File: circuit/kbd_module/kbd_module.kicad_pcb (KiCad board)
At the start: 2 copper layers, 50 x 50 mm, 25 parts, among them SW1 SW_SIMPLE, SW10 SW_SIMPLE, SW11 SW_SIMPLE, SW12 SW_SIMPLE, SW2 SW_SIMPLE, SW3 SW_SIMPLE, SW4 SW_SIMPLE, SW5 SW_SIMPLE, SW6 SW_SIMPLE, SW7 SW_SIMPLE, SW8 SW_SIMPLE, SW9 SW_SIMPLE, U1 NRF24LE1_PROG

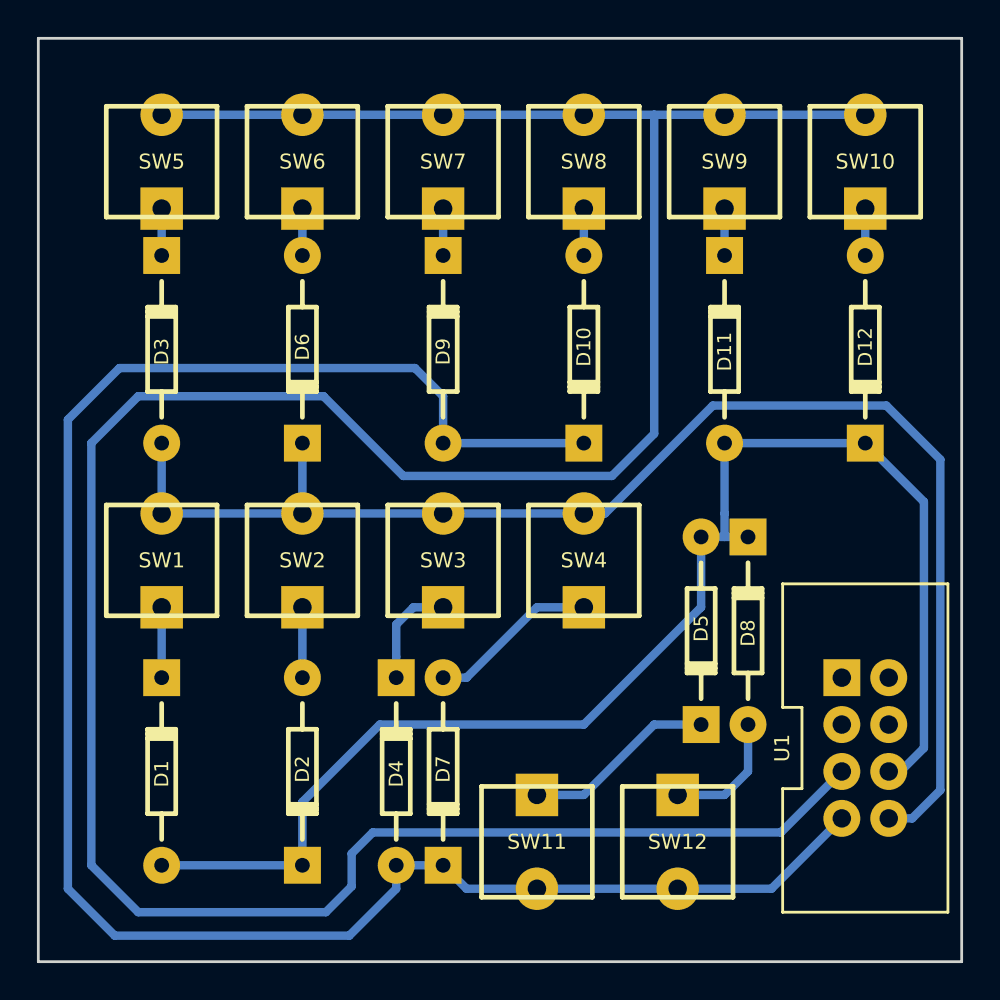
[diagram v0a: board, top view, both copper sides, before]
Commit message: dual diodes
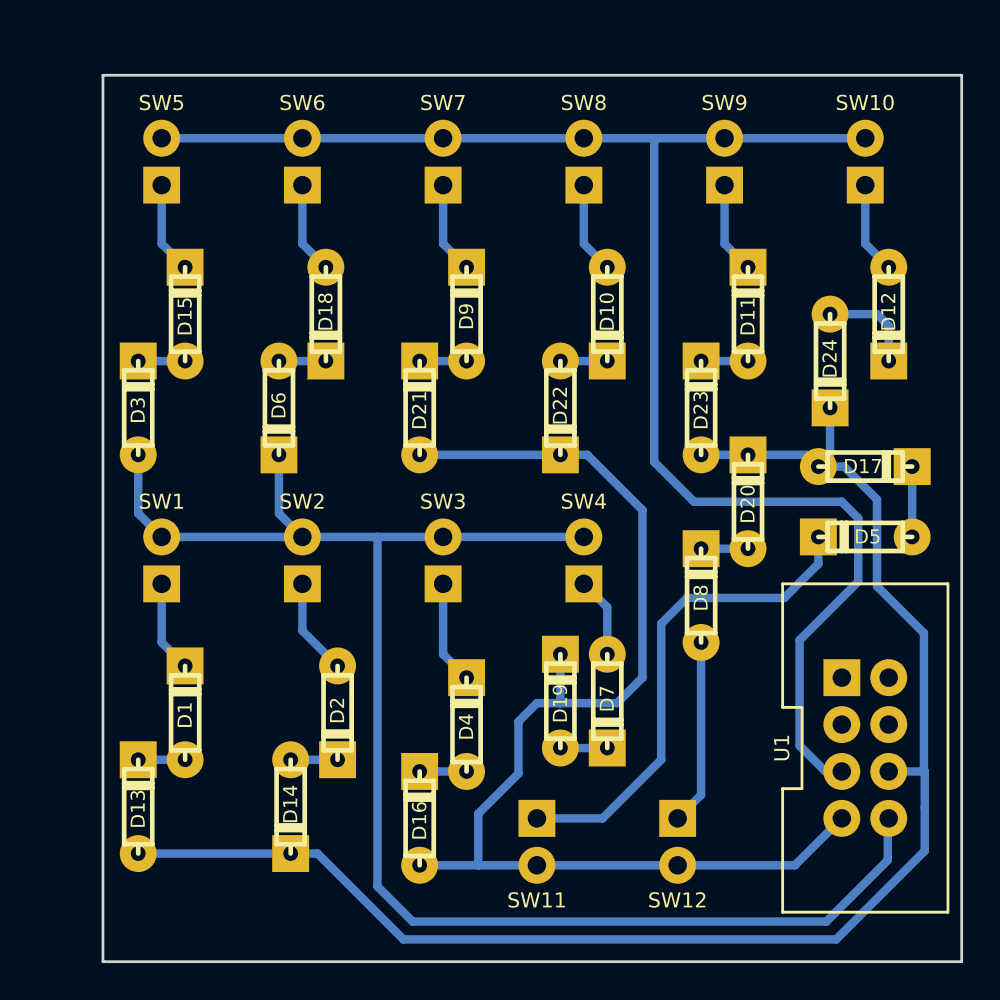
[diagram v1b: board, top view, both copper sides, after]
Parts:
- added D13: 1n4148, kbd_module:SOD27_RM5_5, F.Cu at (105.4, 141.6)
- added D14: 1n4148, kbd_module:SOD27_RM5_5, F.Cu at (113.7, 141.6)
- added D15: 1n4148, kbd_module:SOD27_RM5_5, F.Cu at (108.0, 114.9)
- added D16: 1n4148, kbd_module:SOD27_RM5_5, F.Cu at (120.7, 142.2)
- added D17: 1n4148, kbd_module:SOD27_RM5_5, F.Cu at (144.8, 123.2)
- added D18: 1n4148, kbd_module:SOD27_RM5_5, F.Cu at (115.6, 114.9)
- added D19: 1n4148, kbd_module:SOD27_RM5_5, F.Cu at (128.3, 135.9)
- added D20: 1n4148, kbd_module:SOD27_RM5_5, F.Cu at (138.4, 125.1)
- added D21: 1n4148, kbd_module:SOD27_RM5_5, F.Cu at (120.7, 120.0)
- added D22: 1n4148, kbd_module:SOD27_RM5_5, F.Cu at (128.3, 120.0)
- added D23: 1n4148, kbd_module:SOD27_RM5_5, F.Cu at (135.9, 120.0)
- added D24: 1n4148, kbd_module:SOD27_RM5_5, F.Cu at (142.9, 117.5)
- D1, D10, D11, D12, D2, D3, D4, D5, D6, D7, D8, D9: value D -> 1n4148; footprint kbd_module:Diode_DO-35_SOD27_Horizontal_RM10 -> kbd_module:SOD27_RM5_5
- SW1, SW10, SW11, SW12, SW2, SW3, SW4, SW5, SW6, SW7, SW8, SW9: footprint kbd_module:Tact_6x6 -> kbd_module:ExtSwitch
- moved D5 10.2 mm to (144.8, 127.0), turned to 180 degrees
- moved D7 9.67 mm to (130.8, 135.9)
- moved D4 4.58 mm to (123.2, 137.2)
- moved D2 3.70 mm to (116.2, 136.5)
- moved D3 3.42 mm to (105.4, 120.0)
- moved D6 3.42 mm to (113.0, 120.0)
- moved D1 3.42 mm to (108.0, 136.5)
- moved D8 3.18 mm to (135.9, 130.2)
- moved D10 2.29 mm to (130.8, 114.9)
- moved D11 2.29 mm to (138.4, 114.9)
- moved D12 2.29 mm to (146.1, 114.9)
- moved D9 2.29 mm to (123.2, 114.9)
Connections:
- D1 pad 2: /FMOSI -> Net-(D1-Pad2)
- D10 pad 1: /FMISO -> Net-(D10-Pad1)
- D11 pad 2: /FMOSI -> Net-(D11-Pad2)
- D12 pad 1: /FMOSI -> Net-(D12-Pad1)
- D2 pad 1: /FMOSI -> Net-(D14-Pad2)
- D3 pad 1: Net-(D3-Pad1) -> Net-(D15-Pad2)
- D4 pad 2: /FMISO -> Net-(D16-Pad1)
- D5 pad 2: /FMOSI -> Net-(D17-Pad1)
- D6 pad 2: Net-(D6-Pad2) -> Net-(D18-Pad1)
- D7 pad 1: /FMISO -> Net-(D19-Pad2)
- D8 pad 1: /FMOSI -> Net-(D20-Pad2)
- D9 pad 2: /FMISO -> Net-(D21-Pad1)
- SW5 pad 1: Net-(D3-Pad1) -> Net-(D15-Pad1)
- SW6 pad 1: Net-(D6-Pad2) -> Net-(D18-Pad2)
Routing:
- net /FSCK: track 158.4 -> 84.4 mm
- net /FMISO: track 105.1 -> 65.3 mm
- net Net-(D5-Pad1): track 10.5 -> 26.7 mm
- net /FCSN: track 74.7 -> 83.8 mm
- net /FMOSI: track 76.3 -> 82.5 mm
- net Net-(D12-Pad1): track 0.00 -> 5.34 mm
- net Net-(D18-Pad2): track 0.00 -> 4.97 mm
- net Net-(D15-Pad1): track 0.00 -> 4.97 mm
- net Net-(D7-Pad2): track 9.20 -> 4.34 mm
- net Net-(D17-Pad1): track 0.00 -> 3.81 mm
- net Net-(D8-Pad2): track 6.88 -> 10.1 mm
- net Net-(D20-Pad2): track 0.00 -> 2.54 mm
- net Net-(D11-Pad2): track 0.00 -> 2.54 mm
- net Net-(D6-Pad2): track 2.54 -> 0.00 mm
- net Net-(D3-Pad1): track 2.54 -> 0.00 mm
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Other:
- board size 50 x 50 mm -> 46.5 x 48 mm
